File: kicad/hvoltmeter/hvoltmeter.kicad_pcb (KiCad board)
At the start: 2 copper layers, 14.4 x 24.9 mm, 35 parts, among them J1 USB_B_Micro-Connector, J2 SWC, J3 SWD, J4 Conn, J5 Conn, J6 Conn, SW1 SW_DPDT_x2, U1 LTC4054ES5-4.2, U2 AD8541, U3 MCP1700

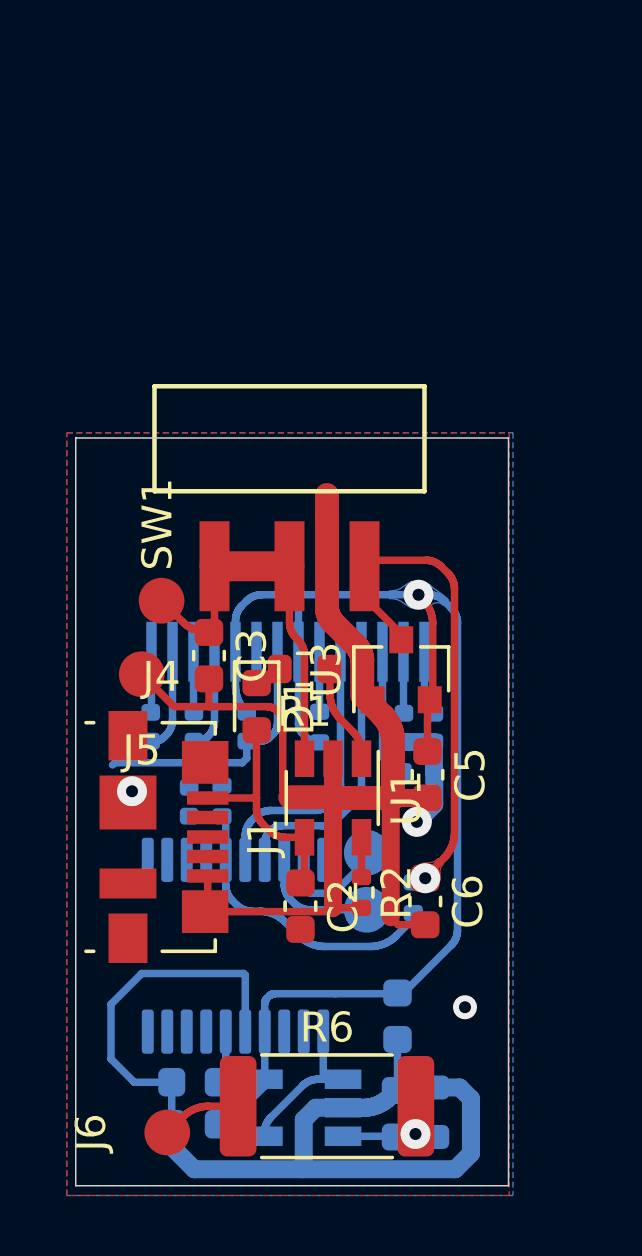
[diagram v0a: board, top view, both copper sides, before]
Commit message: изменено:      kicad/hvoltmeter/hvoltmeter.kicad_pcb 	изменено:      kicad/hvoltmeter/hvoltmeter.kicad_pcb-bak
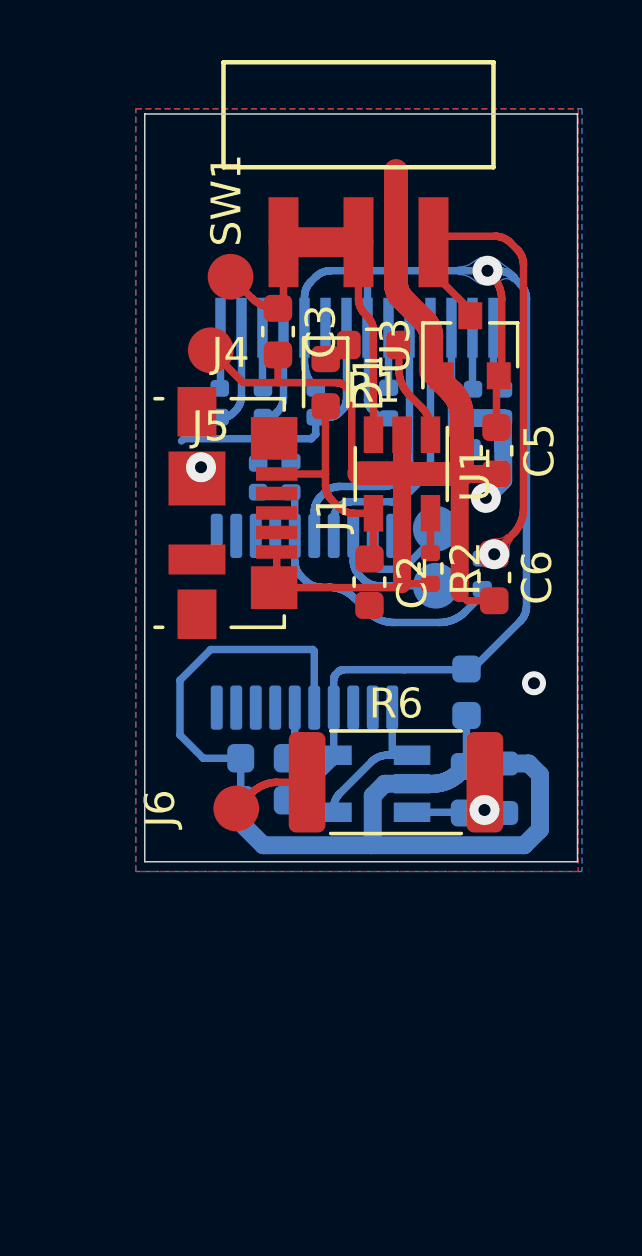
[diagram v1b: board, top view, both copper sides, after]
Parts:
- moved C1 11.0 mm to (42.3, 64.6)
- moved R5 11.0 mm to (50.3, 65.6)
- moved C2 11.0 mm to (45.8, 58.7)
- moved C4 11.0 mm to (49.0, 62.4)
- moved C5 11.0 mm to (50.0, 54.4)
- moved D1 11.0 mm to (44.3, 52.1)
- moved J3 11.0 mm to (48.0, 58.9)
- moved J4 11.0 mm to (41.2, 48.5)
- moved R2 11.0 mm to (47.8, 58.3)
- moved R4 11.0 mm to (43.2, 55.2)
- moved R8 11.0 mm to (46.4, 52.8)
- moved SW1 11.0 mm to (45.4, 45.9)
- moved C10 11.0 mm to (49.2, 52.8)
- moved C11 11.0 mm to (40.8, 52.8)
- moved C12 11.0 mm to (42.2, 52.8)
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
